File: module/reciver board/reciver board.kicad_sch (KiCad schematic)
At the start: 23 parts, among them U1 LTC4316xDD, U10 LTC4316xDD, U11 LTC4316xDD, U12 LTC4316xDD, U16 OSMC Module Board, U17 OSMC Module Board, U18 OSMC Module Board, U19 OSMC Module Board, U2 OSMC Module Board, U20 OSMC Module Board, U21 OSMC Module Board, U3 24LC32, U4 OSMC Module Board, U7 24AA02-OT, U9 LTC4316xDD

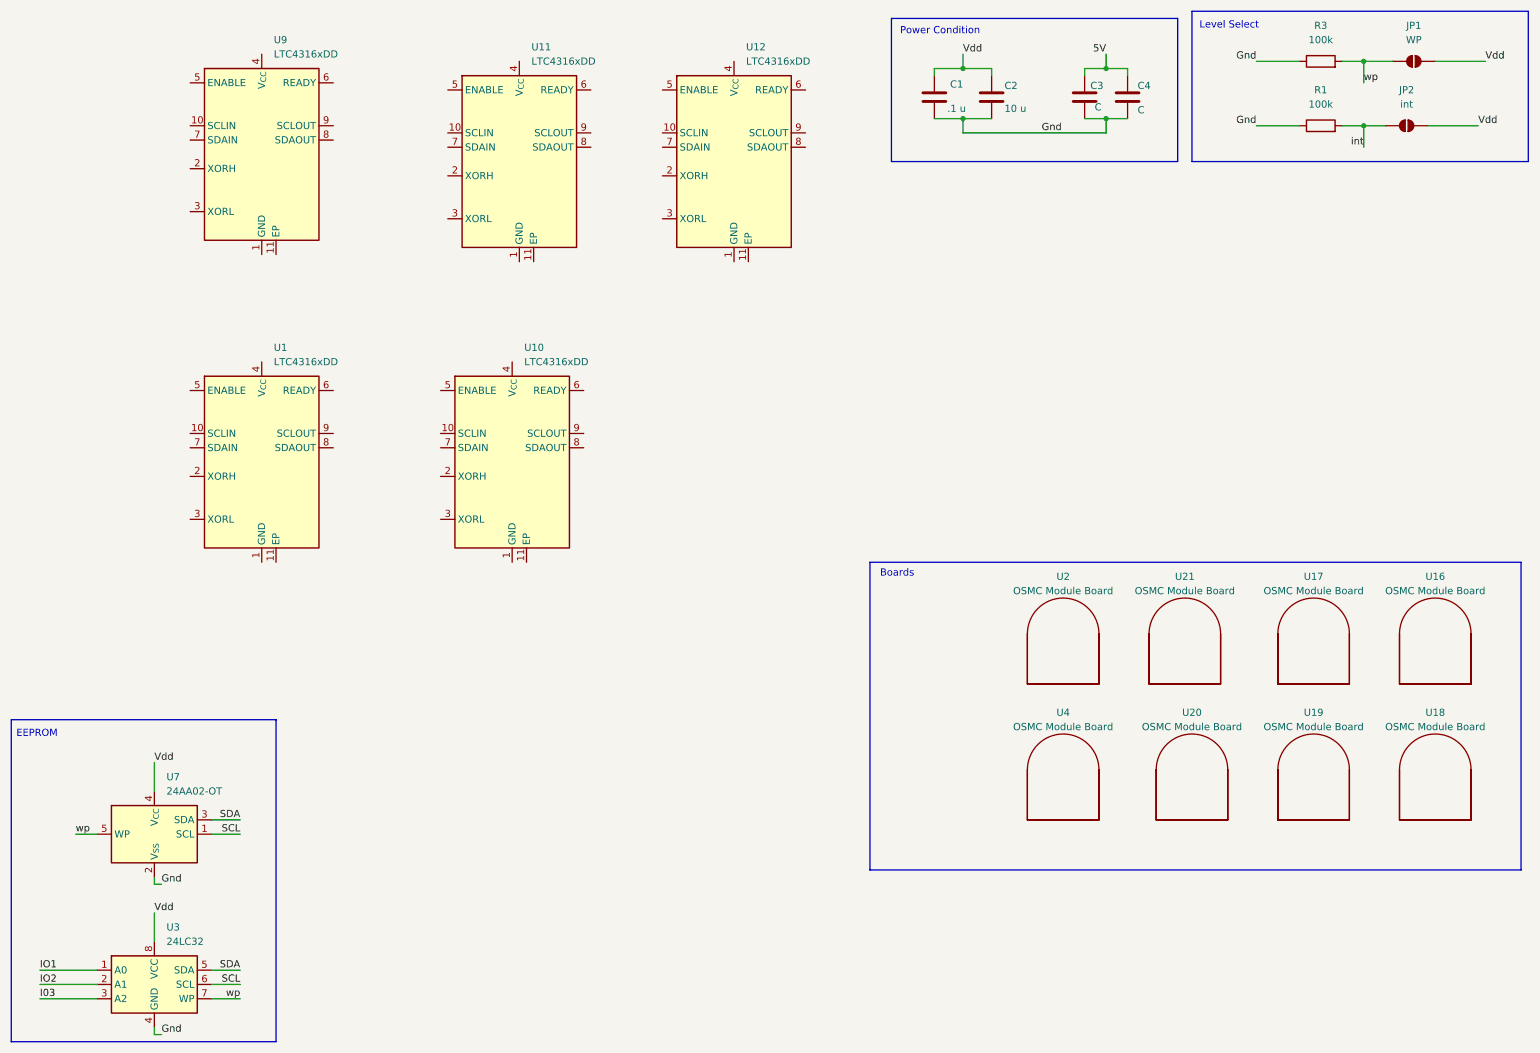
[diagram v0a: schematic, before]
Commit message: update
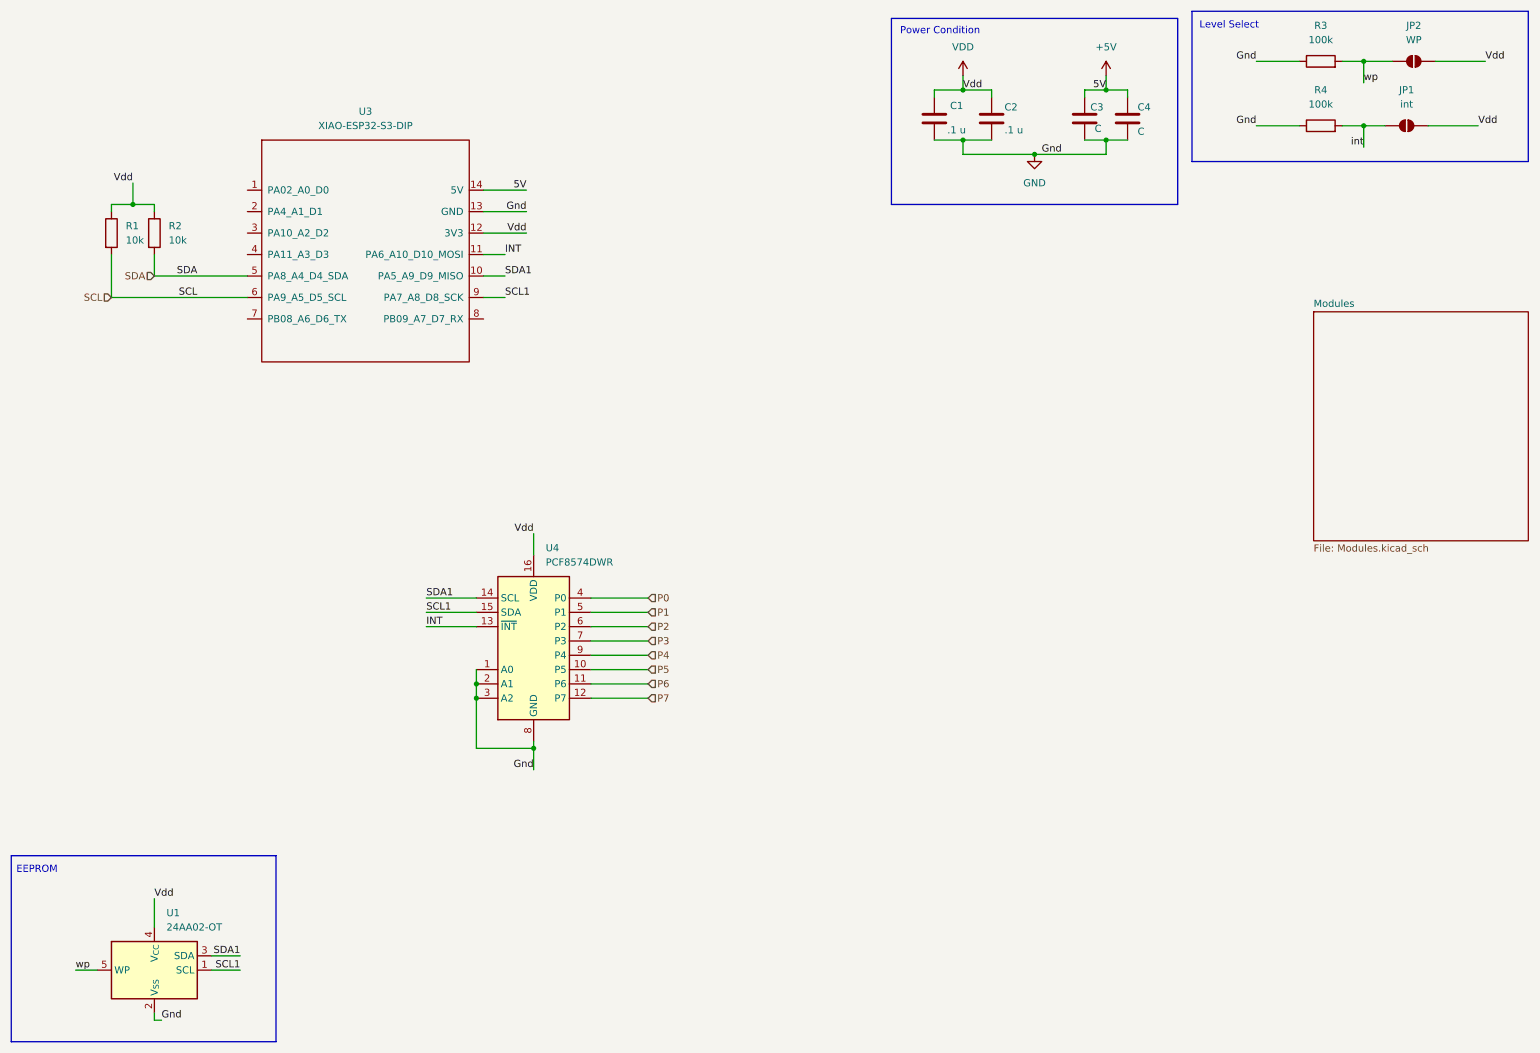
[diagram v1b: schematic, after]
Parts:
- removed U1, U10, U11, U12, U9: LTC4316xDD, Package_DFN_QFN:DFN-10-1EP_3x3mm_P0.5mm_EP1.65x2.38mm, symbol Interface_Expansion:LTC4316xDD
- removed U16, U17, U18, U19, U2, U20, U21, U4: OSMC Module Board, OSMC_Module:Module standard v2, symbol OSMC_Module:Input_Module_Pinless
- removed U3: 24LC32, Package_SO:SOIC-8_3.9x4.9mm_P1.27mm, symbol Memory_EEPROM:24LC32
- added R1, R2: 10k, symbol Library:R
- added U3: XIAO-ESP32-S3-DIP, Seed Studio Xiao:XIAO-ESP32-S3-DIP, symbol Library:XIAO-ESP32-S3-DIP
- added U4: PCF8574DWR, PCF8574DWR:DW16-L, symbol Library:PCF8574AT
- C1, C3, C4: symbol Device:C -> Library:C
- C2: value 10 u -> .1 u; symbol Device:C -> Library:C
- JP1: renamed from JP2; symbol Jumper:SolderJumper_2_Open -> Library:SolderJumper_2_Open
- JP2: renamed from JP1; symbol Jumper:SolderJumper_2_Open -> Library:SolderJumper_2_Open
- R3: symbol Device:R -> Library:R
- R4: renamed from R1; symbol Device:R -> Library:R
- U1: renamed from U7; footprint Package_TO_SOT_SMD:SOT-23-5_HandSoldering -> Package_TO_SOT_SMD:SOT-23-5; symbol Memory_EEPROM:24AA02-OT -> Library:24AA02-OT
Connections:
- net SCL: now also R1.2, U3.6 (PA9_A5_D5_SCL); no longer U1.1 (SCL)
- net SDA: now also R2.2, U3.5 (PA8_A4_D4_SDA); no longer U1.3 (SDA)
- net 5V renamed +5V
- net +5V: now also U3.14 (5V)
- net Gnd renamed GND
- net GND: now also U3.13 (GND), U4.1 (A0), U4.2 (A1), U4.3 (A2), U4.8 (GND)
- net Vdd renamed VDD
- net VDD: now also R1.1, R2.1, U3.12 (3V3), U4.16 (VDD)
- new net INT: U3.11 (PA6_A10_D10_MOSI), U4.13 (~{INT})
- new net P0: U4.4 (P0)
- new net P1: U4.5 (P1)
- new net P2: U4.6 (P2)
- new net P3: U4.7 (P3)
- new net P4: U4.9 (P4)
- new net P5: U4.10 (P5)
- new net P6: U4.11 (P6)
- new net P7: U4.12 (P7)
- new net SCL1: U1.1 (SCL), U3.9 (PA7_A8_D8_SCK), U4.15 (SDA)
- new net SDA1: U1.3 (SDA), U3.10 (PA5_A9_D9_MISO), U4.14 (SCL)
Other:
- added sheet Modules (Modules.kicad_sch)
- note removed: "Boards"
- moved on the sheet: C1, C2, C3, C4, U1

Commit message: update
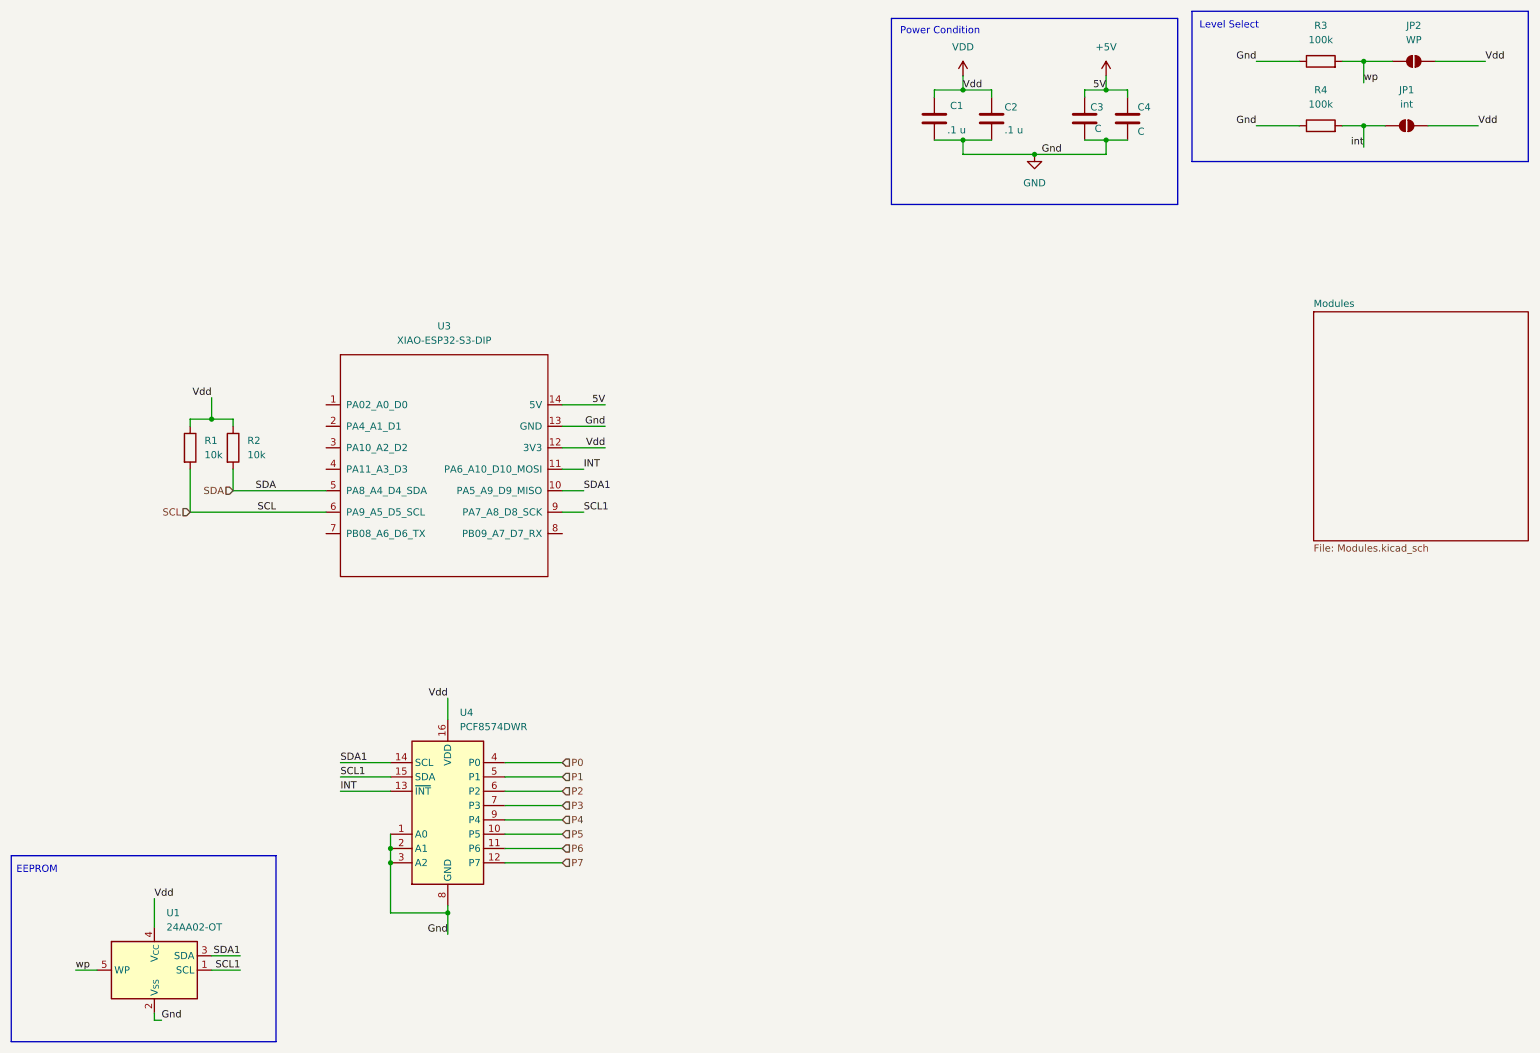
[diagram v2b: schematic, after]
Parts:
- R3, R4: footprint PCM_Resistor_SMD_AKL:R_0805_2012Metric_Pad1.15x1.40mm_HandSolder -> PCM_Resistor_SMD_AKL:R_0603_1608Metric_Pad1.05x0.95mm_HandSolder
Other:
- moved on the sheet: R1, R2, U3, U4
